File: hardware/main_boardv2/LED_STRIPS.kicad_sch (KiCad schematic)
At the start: 8 parts, among them IC801 SN74LV1T34DBVR, J802 Conn_01x03_Pin

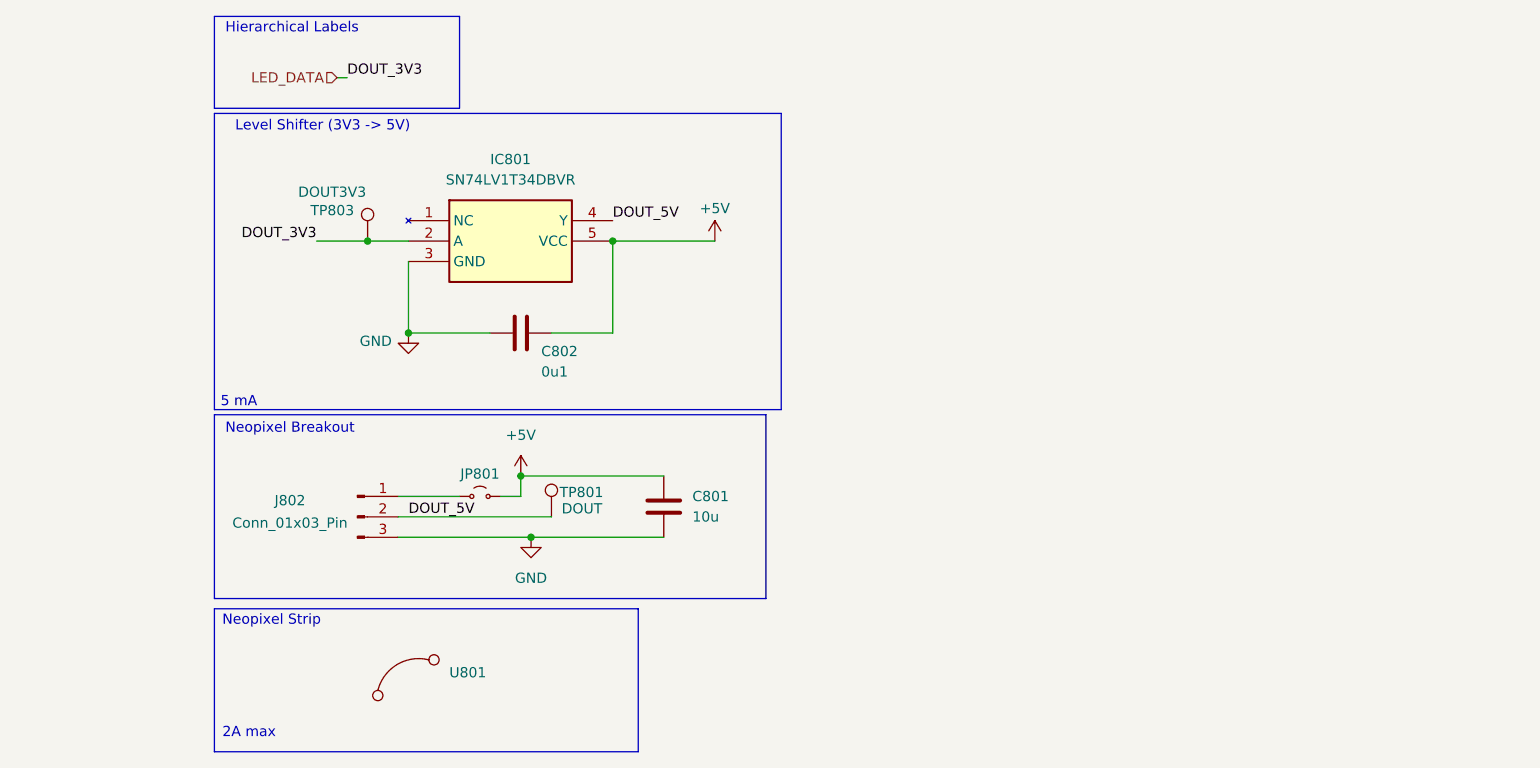
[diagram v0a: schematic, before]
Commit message: more hardware
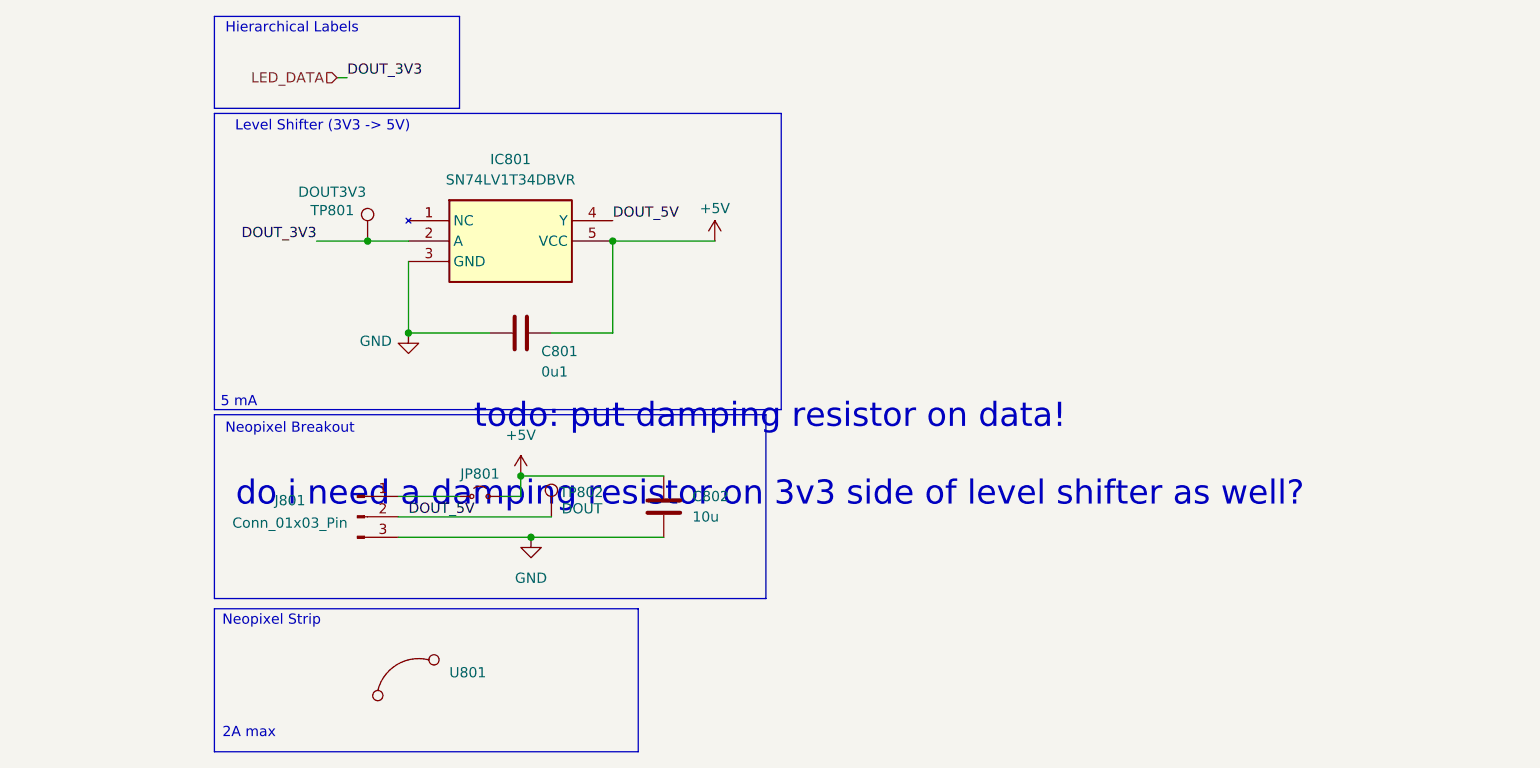
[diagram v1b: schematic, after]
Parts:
- renumbered C802 to C801, C801 to C802, J802 to J801, TP803 to TP801, TP801 to TP802
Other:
- note added: "todo: put damping resistor on data! do i need a damping resistor on 3v3 side of level shifter as well?"
